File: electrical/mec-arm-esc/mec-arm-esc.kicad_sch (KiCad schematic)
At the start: 0 parts

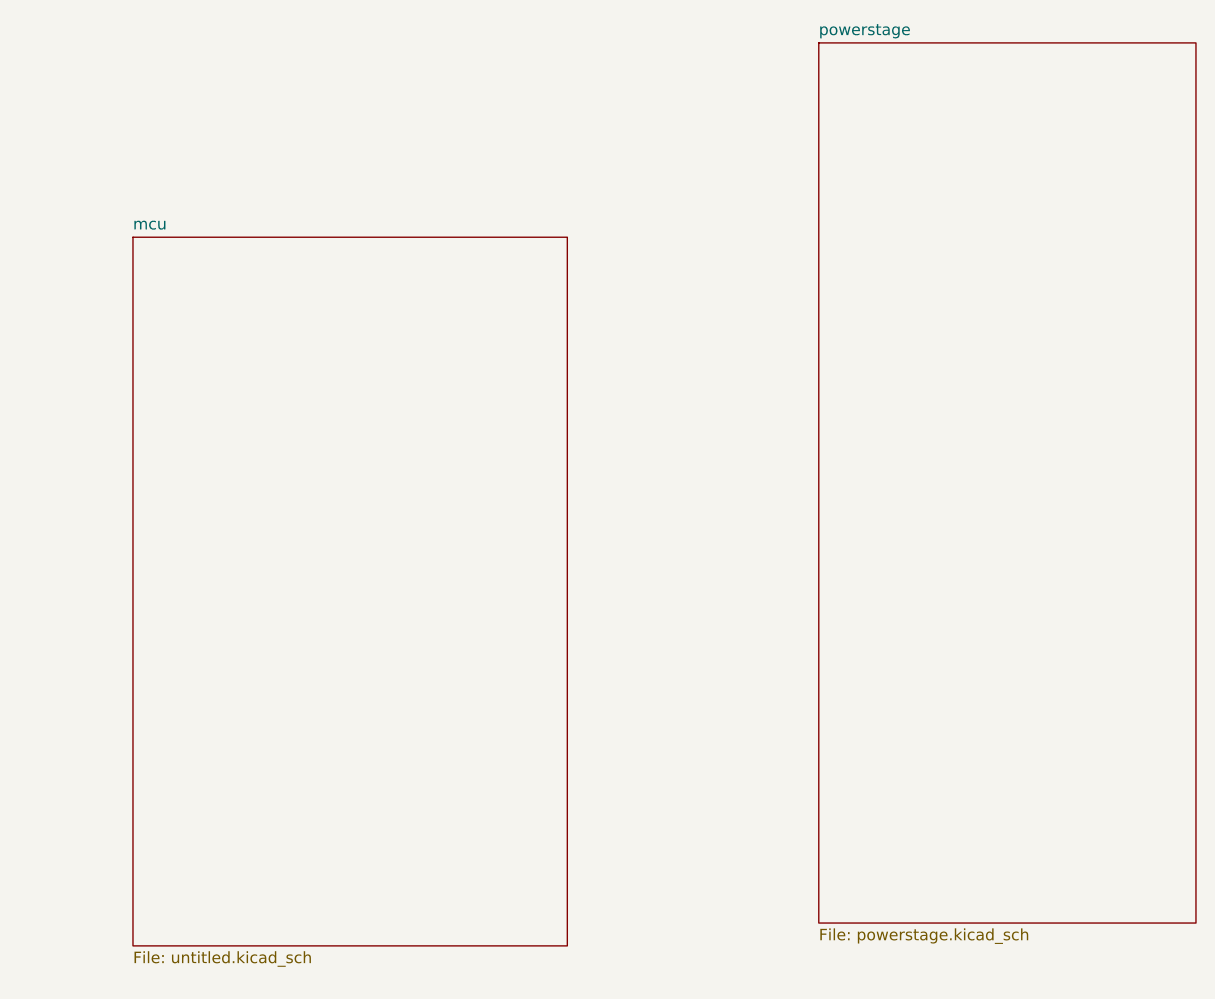
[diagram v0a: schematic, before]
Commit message: added backups
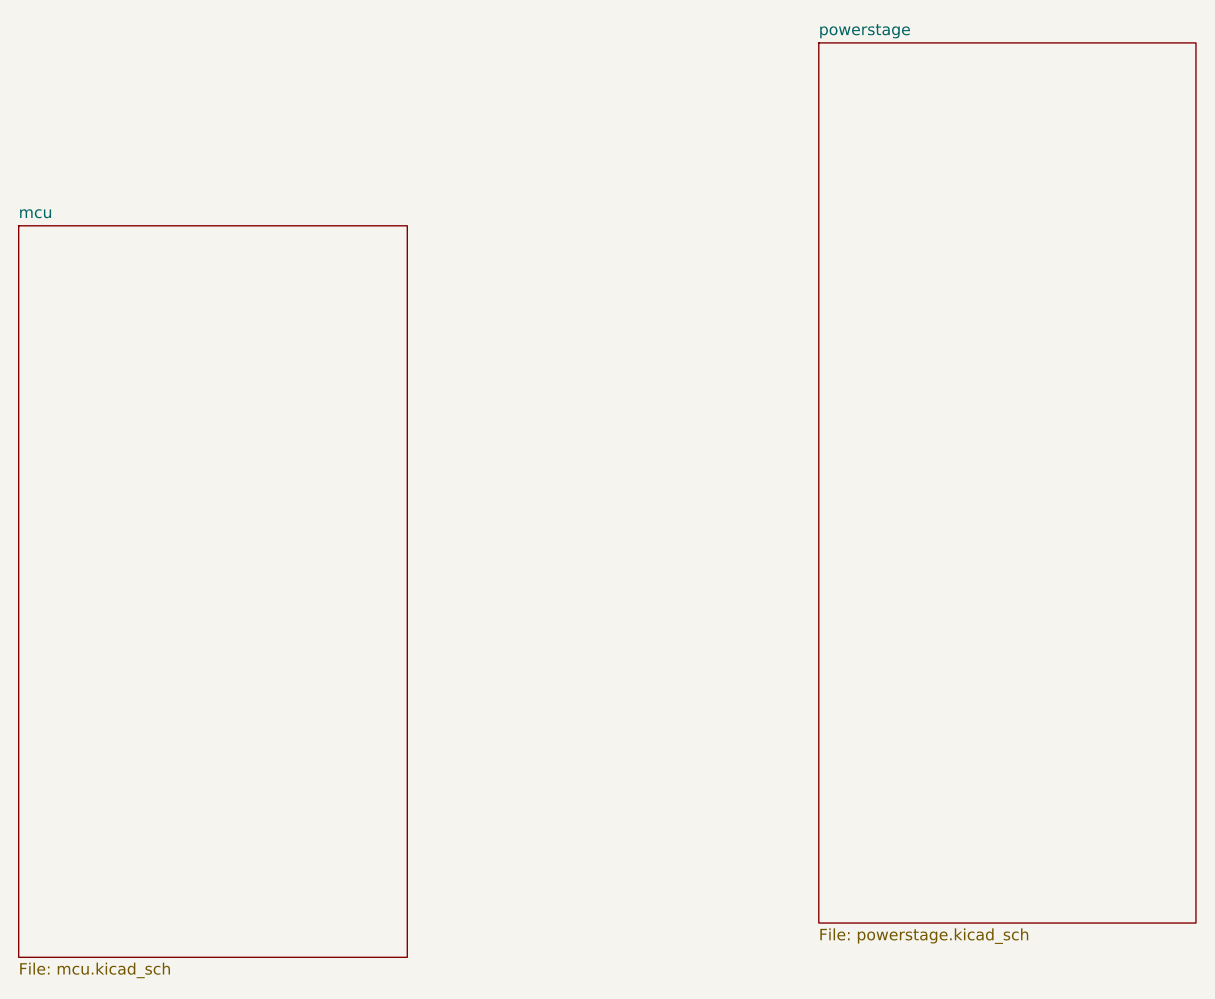
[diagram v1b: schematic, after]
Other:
- sheet mcu: file untitled.kicad_sch -> mcu.kicad_sch
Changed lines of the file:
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@@
 	)
 	(sheet
-		(at 127 60.96)
-		(size 48.26 78.74)
+		(at 114.3 59.69)
+		(size 43.18 81.28)
 		(exclude_from_sim no)
 		(in_bom yes)
@@
 		)
 		(fill
-			(color 110 124 255 1)
+			(color 0 0 0 0)
 		)
 		(property "Sheetname" "mcu"
-			(at 127 60.2484 0)
+			(at 114.3 58.9784 0)
 			(show_name no)
 			(do_not_autoplace no)
@@
 			)
 		)
-		(property "Sheetfile" "untitled.kicad_sch"
-			(at 127 140.2846 0)
+		(property "Sheetfile" "mcu.kicad_sch"
+			(at 114.3 141.5546 0)
 			(show_name no)
 			(do_not_autoplace no)
